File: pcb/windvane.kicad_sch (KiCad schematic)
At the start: 0 parts

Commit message: schematic done, next up - layout
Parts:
- added C1, C2: 22u, Capacitor_SMD:C_Elec_5x5.8, symbol Device:C_Polarized_Small
- added C3, C6, C7: 0.1u, Capacitor_SMD:C_0805_2012Metric, symbol Device:C
- added C4, C5: 22p, Capacitor_SMD:C_0805_2012Metric, symbol Device:C
- added H1, H2, H3, H4: MountingHole, MountingHole:MountingHole_2.2mm_M2, symbol Mechanical:MountingHole
- added J1: Screw_Terminal_01x04, TerminalBlock_Phoenix:TerminalBlock_Phoenix_MKDS-1,5-4-5.08_1x04_P5.08mm_Horizontal, symbol Connector:Screw_Terminal_01x04
- added J2: Conn_01x04_Pin, Connector_JST:JST_EH_S4B-EH_1x04_P2.50mm_Horizontal, symbol Connector:Conn_01x04_Pin
- added R1, R10, R2, R3, R4, R5, R6, R7, R8, R9: 10k, Resistor_SMD:R_0805_2012Metric, symbol Device:R
- added SS40AF1: ~, Package_TO_SOT_THT:TO-92L_Inline, symbol custom:SS40AF
- added U1: ESP-12F, RF_Module:ESP-12E, symbol RF_Module:ESP-12F
- added U2: MCP2515-xSO, Package_SO:SOIC-18W_7.5x11.6mm_P1.27mm, symbol Interface_CAN_LIN:MCP2515-xSO
- added U3: AS5600-ASOT, Package_SO:Infineon_PG-DSO-8-43, symbol Sensor_Magnetic:AS5600
- added U4: DS18B20, Package_TO_SOT_THT:TO-92_Inline, symbol Sensor_Temperature:DS18B20
- added U5: ~, symbol custom:MiniStepDownConverter
- added U6: TJA1050, Package_SO:SOIC-8_3.9x4.9mm_P1.27mm, symbol custom:TJA1050
- added Y1: 8MHz, Crystal:Crystal_HC49-4H_Vertical, symbol Device:Crystal
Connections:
- new net: C5.2, U2.7 (OSC2), Y1.1
- new net: C4.2, U2.8 (OSC1), Y1.2
- new net: R7.2, U1.17 (GPIO2)
- new net: U2.1 (TXCAN), U6.1 (TXD)
- new net: U2.2 (RXCAN), U6.4 (RXD)
- new net: C3.1, R1.2, U1.1 (~{RST})
- new net: R2.2, U1.3 (EN)
- new net: R10.2, U2.17 (~{RESET})
- new net: R8.1, U1.16 (GPIO15)
- new net +12V: C1.1, J1.4 (Pin_4), SS40AF1.1 (Vs), U5.1 (IN+)
- new net +3V3: C2.1, C6.2, C7.2, R1.1, R10.1, R2.1, R3.1, R4.1, R5.1, R6.1, R7.1, R9.1, U1.8 (VCC), U2.18 (VDD), U3.1 (VDD5V), U3.2 (VDD3V3), U4.3 (V_{DD}), U5.3 (OUT+), U6.3 (VCC)
- new net CAN_HI: J1.2 (Pin_2), U6.7 (CANH)
- new net CAN_LOW: J1.1 (Pin_1), U6.6 (CANL)
- new net CAN_~{Int}: U1.4 (GPIO16), U2.12 (~{INT})
- new net GND: C1.2, C2.2, C3.2, C4.1, C5.1, C6.1, C7.1, J1.3 (Pin_3), J2.4 (Pin_4), R8.2, SS40AF1.3 (GND), U1.15 (GND), U2.9 (VSS), U3.4 (GND), U3.8 (DIR), U4.1 (GND), U5.2 (GND), U5.4 (GND), U6.2 (GND), U6.8 (S)
- new net MISO: U1.10 (MISO), U2.15 (SO)
- new net MOSI: U1.13 (MOSI), U2.14 (SI)
- new net SCL: R5.2, U1.20 (GPIO5), U3.7 (SCL)
- new net SCLK: U1.14 (SCLK), U2.13 (SCK)
- new net SDA: R4.2, U1.19 (GPIO4), U3.6 (SDA)
- new net Speed_Out: SS40AF1.2 (Out), U1.5 (GPIO14)
- new net Temp_DQ: R3.2, R9.2, U1.6 (GPIO12), U4.2 (DQ)
- new net uC_PRG: J2.1 (Pin_1), R6.2, U1.18 (GPIO0)
- new net uC_RXD: J2.3 (Pin_3), U1.21 (GPIO3/RXD)
- new net uC_TXD: J2.2 (Pin_2), U1.22 (GPIO1/TXD)
- new net ~{CS}: U1.12 (GPIO10), U2.16 (~{CS})
- no-connect marks 0 -> 13
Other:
- note added: "CAN/NMEA200 interface"
- note added: "Controller"
- note added: "Direction sensor"
- note added: "Input/Output"
- note added: "Power supply"
- note added: "Speed sensor"
- note added: "Temperature sensor"

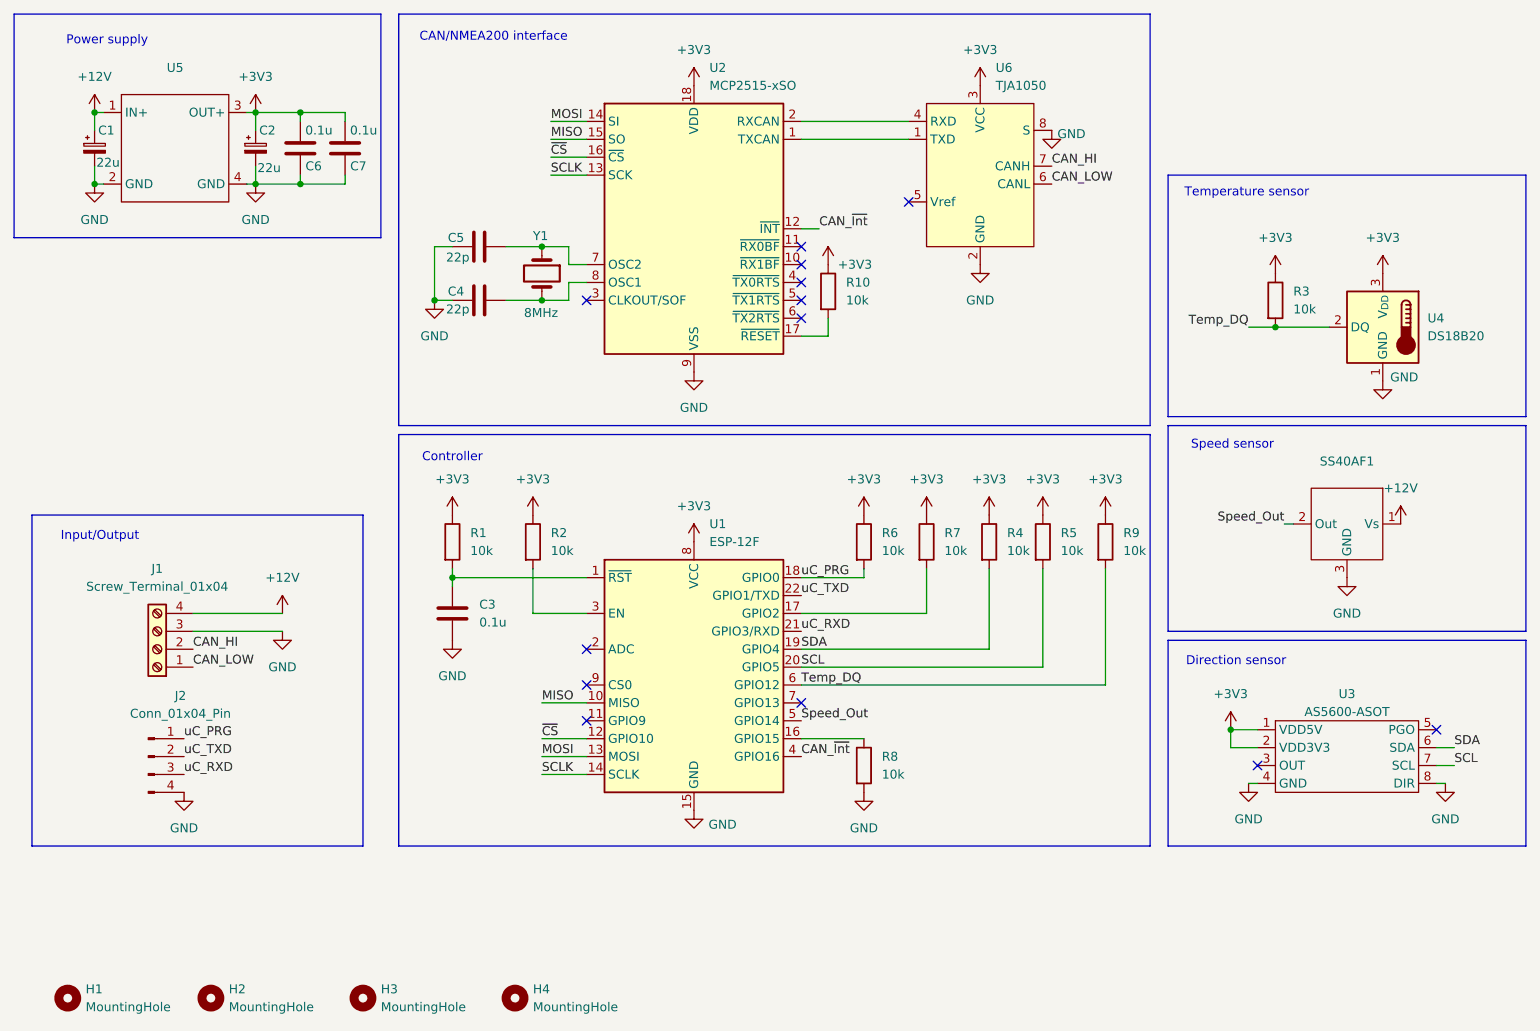
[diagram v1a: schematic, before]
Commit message: place & route
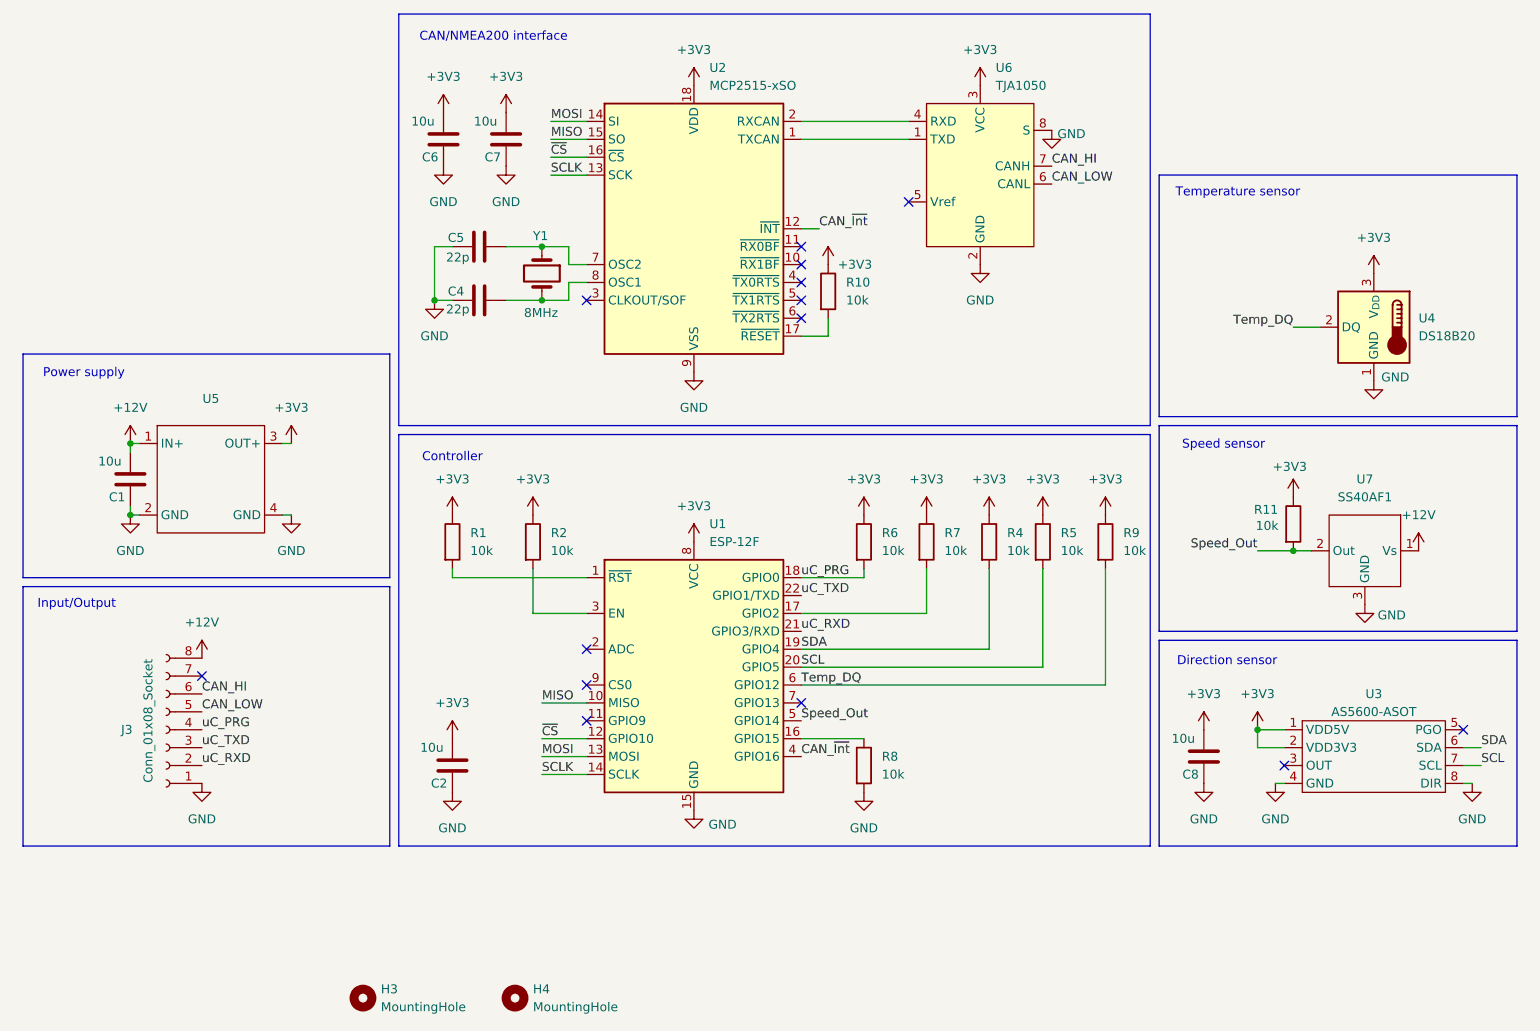
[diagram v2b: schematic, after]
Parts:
- removed C1, C2: 22u, Capacitor_SMD:C_Elec_5x5.8, symbol Device:C_Polarized_Small
- removed C3: 0.1u, Capacitor_SMD:C_0805_2012Metric, symbol Device:C
- removed H1, H2: MountingHole, MountingHole:MountingHole_2.2mm_M2, symbol Mechanical:MountingHole
- removed J1: Screw_Terminal_01x04, TerminalBlock_Phoenix:TerminalBlock_Phoenix_MKDS-1,5-4-5.08_1x04_P5.08mm_Horizontal, symbol Connector:Screw_Terminal_01x04
- removed J2: Conn_01x04_Pin, Connector_JST:JST_EH_S4B-EH_1x04_P2.50mm_Horizontal, symbol Connector:Conn_01x04_Pin
- removed R3: 10k, Resistor_SMD:R_0805_2012Metric, symbol Device:R
- added C1, C2, C8: 10u, Capacitor_SMD:C_0805_2012Metric, symbol Device:C
- added J3: Conn_01x08_Socket, Connector_FFC-FPC:Molex_200528-0080_1x08-1MP_P1.00mm_Horizontal, symbol Connector:Conn_01x08_Socket
- added R11: 10k, Resistor_SMD:R_0805_2012Metric, symbol Device:R
- C6, C7: value 0.1u -> 10u
- U3: footprint Package_SO:Infineon_PG-DSO-8-43 -> Package_SO:SOIC-8_3.9x4.9mm_P1.27mm
- U5: footprint (none) -> Custom:MiniStepDownConverter
- U7: renamed from SS40AF1; value ~ -> SS40AF1
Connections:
- net +12V: now also C1.2, J3.8 (Pin_8)
- net +3V3: now also C2.2, C8.2, R11.1
- net CAN_HI: now also J3.6 (Pin_6)
- net CAN_LOW: now also J3.5 (Pin_5)
- net GND: now also C1.1, C2.1, C8.1, J3.1 (Pin_1)
- net Speed_Out: now also R11.2
- net uC_PRG: now also J3.4 (Pin_4)
- net uC_RXD: now also J3.2 (Pin_2)
- net uC_TXD: now also J3.3 (Pin_3)
- no-connect marks 13 -> 14
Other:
- moved on the sheet: U3, U4, U5, U7
